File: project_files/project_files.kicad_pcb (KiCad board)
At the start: 2 copper layers, 142.9 x 95.2 mm, 27 parts, among them SW11 SW_Push, SW12 SW_Push, SW13 SW_Push, SW17 SW_Push, SW18 SW_Push, SW19 SW_Push, SW3 SW_Push, SW4 SW_Push, SW5 SW_Push, SW7 SW_Push, SW8 SW_Push, SW9 SW_Push, U1 MOUDLE-SEEEDUINO-XIAO

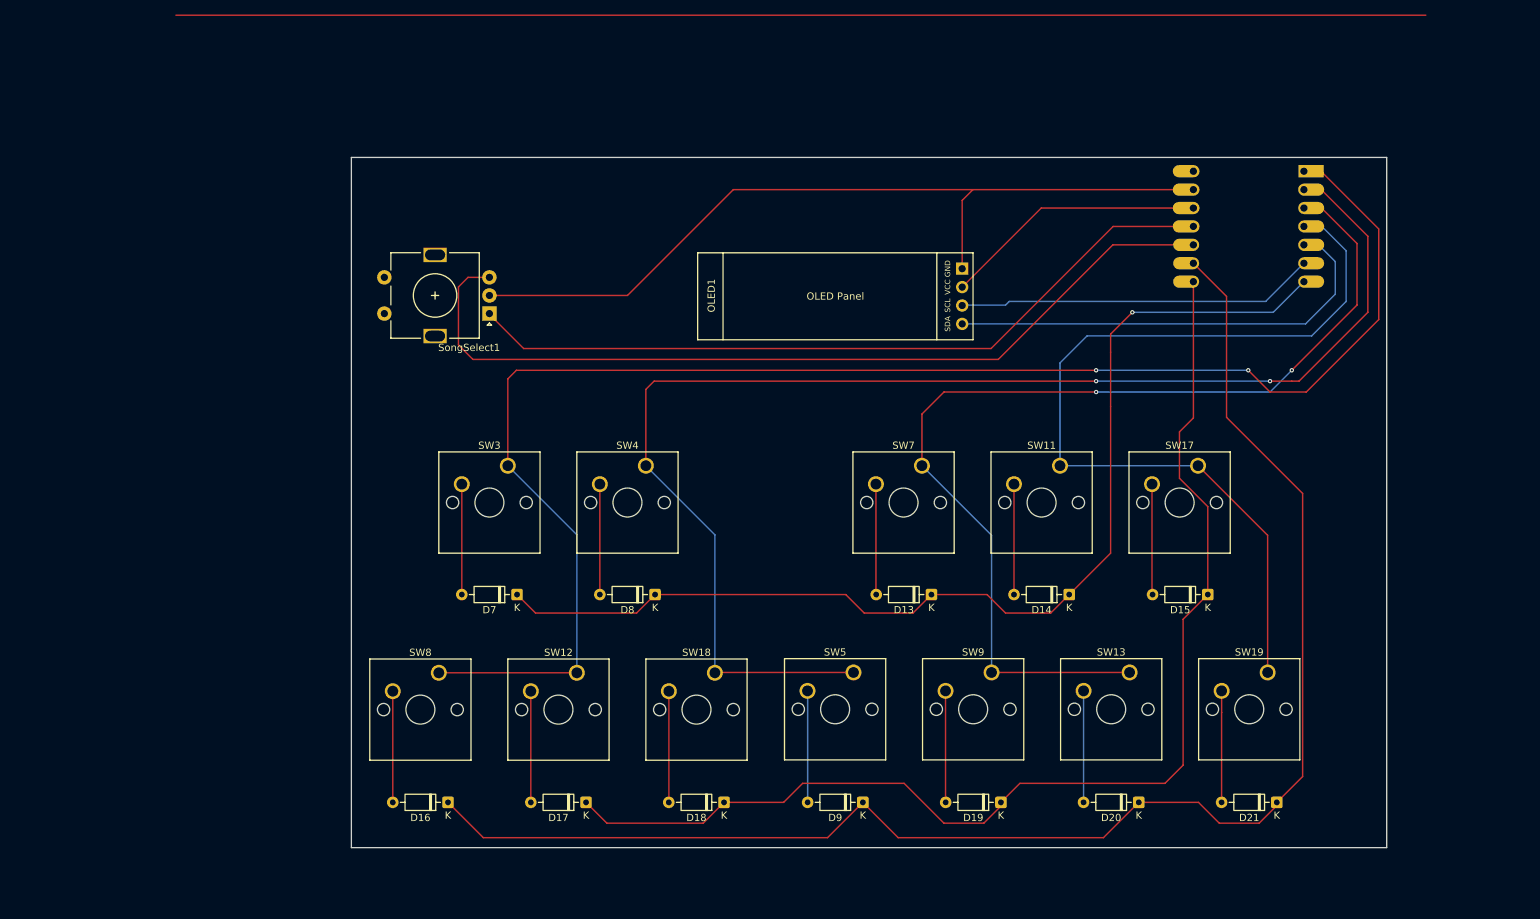
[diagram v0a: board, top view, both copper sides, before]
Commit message: new pcb design
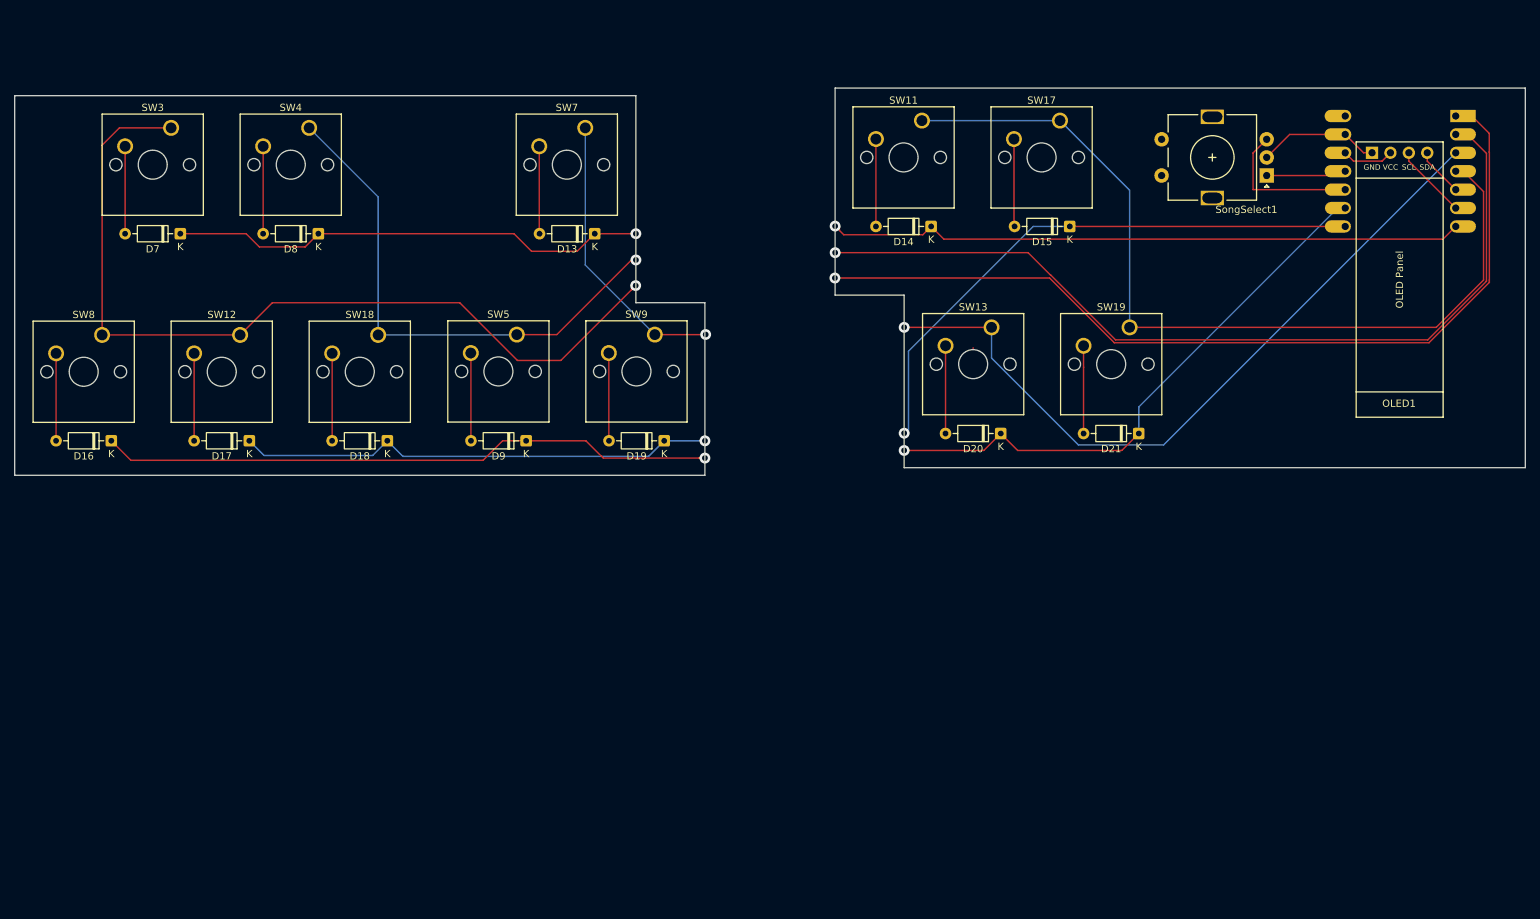
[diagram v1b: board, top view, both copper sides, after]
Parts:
- moved SongSelect1 108.9 mm to (212.0, 50.1)
- moved OLED1 93.7 mm to (224.4, 83.5), turned to 90 degrees
- moved D16 68.2 mm to (52.6, 86.7)
- moved D17 68.2 mm to (71.6, 86.7)
- moved D18 68.2 mm to (90.7, 86.7)
- moved D19 68.2 mm to (128.9, 86.7)
- moved D9 68.2 mm to (109.8, 86.7)
- moved D13 68.1 mm to (119.3, 58.2)
- moved D8 68.1 mm to (81.2, 58.2)
- moved D7 68.1 mm to (62.1, 58.2)
- moved SW12 65.8 mm to (70.4, 72.1)
- moved SW7 65.8 mm to (118.0, 43.5)
- moved SW8 65.8 mm to (51.3, 72.1)
- moved SW9 65.8 mm to (127.6, 72.1)
- moved SW3 65.8 mm to (60.9, 43.5)
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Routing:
- net /PIN_10: track 121.6 -> 21.3 mm
- net GND: track 114.7 -> 16.9 mm
- net /PIN_11: track 106.2 -> 11.2 mm
- net /SDA: track 63.0 -> 6.72 mm
- net /PIN_9: track 207.2 -> 163.2 mm, vias 0 -> 2
- net /SCL: track 49.6 -> 10.3 mm
- net /PWR_3v3: track 36.4 -> 7.19 mm
- net /PIN_1: track 215.7 -> 242.5 mm
- net /PIN_8: track 162.3 -> 145.0 mm, vias 0 -> 2
- net /PIN_2: track 188.2 -> 192.4 mm
- net /PIN_7: track 150.5 -> 154.1 mm, vias 1 -> 2
- net Net-(D21-A): track 15.4 -> 12.1 mm
- net Net-(D17-A): track 15.3 -> 12.1 mm
- net Net-(D16-A): track 15.3 -> 12.1 mm
- net Net-(D19-A): track 15.4 -> 12.1 mm
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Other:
- board size 142.9 x 95.2 mm -> 208.5 x 53.4 mm

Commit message: pcb done maybe
kudos anicetus
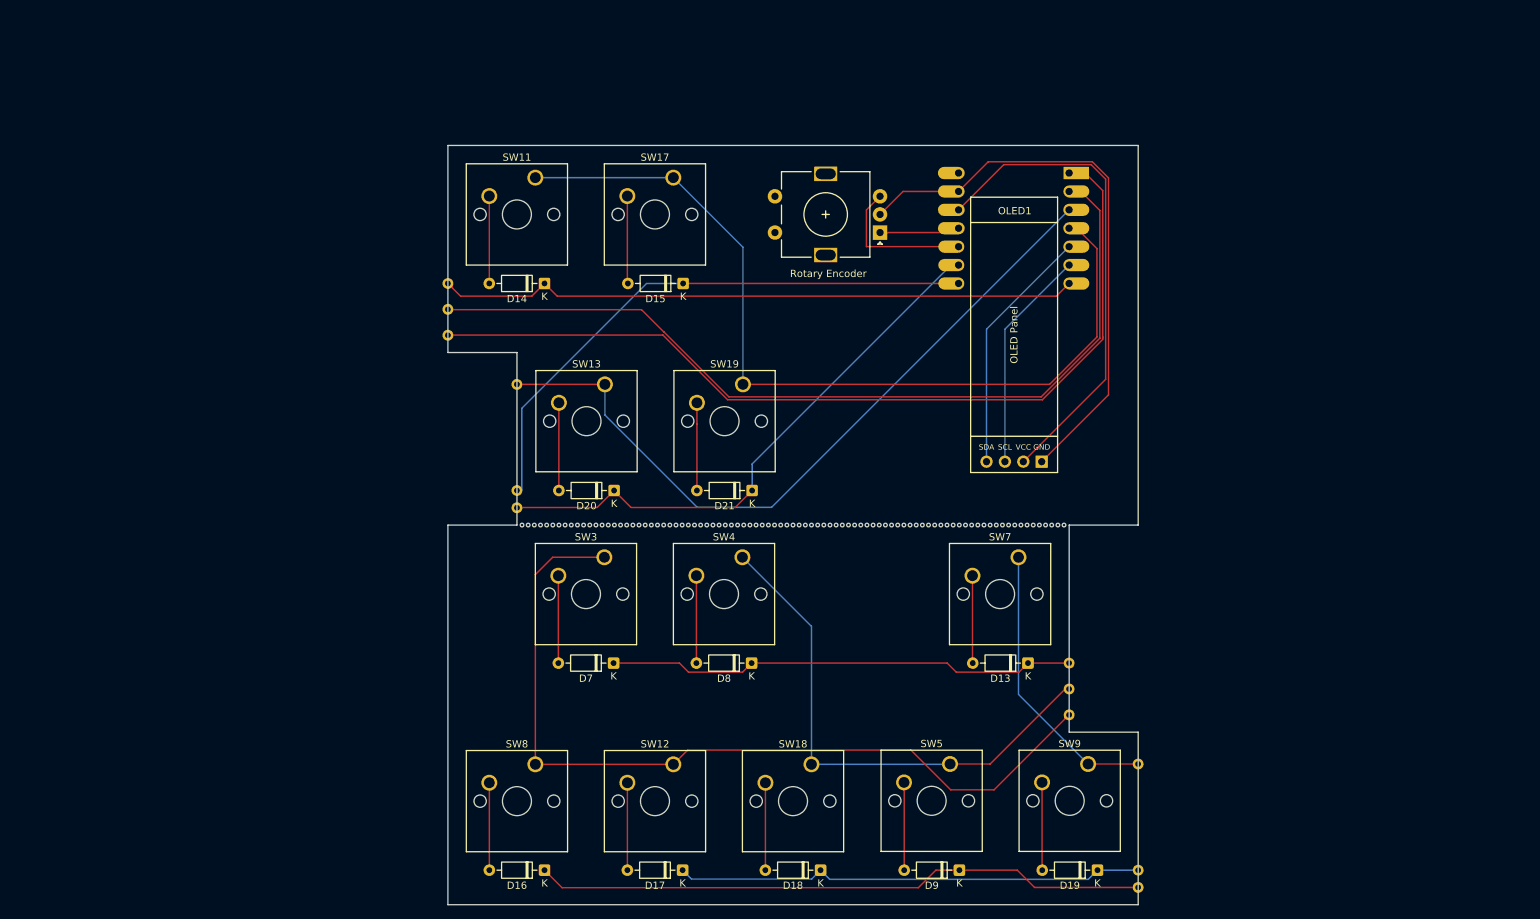
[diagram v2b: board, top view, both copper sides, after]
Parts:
- added ?: , , F.Cu at (99.0, 68.6)
- added ?: , , F.Cu at (108.6, 93.6)
- added ?: , , F.Cu at (108.6, 96.0)
- added ?: , , F.Cu at (194.3, 131.3)
- added ?: , , F.Cu at (184.8, 124.6)
- added ?: , , F.Cu at (194.3, 148.4)
- added ?: , , F.Cu at (99.0, 65.0)
- added ?: , , F.Cu at (184.8, 117.4)
- added ?: , , F.Cu at (194.3, 146.0)
- added ?: , , F.Cu at (184.8, 121.0)
- added ?: , , F.Cu at (108.6, 78.9)
- added ?: , , F.Cu at (99.0, 72.2)
- added REF**: BreakLine_11h_D0.5mm_P0.85mm, Panelization:BreakLine_11h_D0.5mm_P0.85mm, F.Cu at (179.0, 98.4)
- added REF**: BreakLine_11h_D0.5mm_P0.85mm, Panelization:BreakLine_11h_D0.5mm_P0.85mm, F.Cu at (132.2, 98.4)
- added REF**: BreakLine_11h_D0.5mm_P0.85mm, Panelization:BreakLine_11h_D0.5mm_P0.85mm, F.Cu at (113.5, 98.4)
- added REF**: BreakLine_11h_D0.5mm_P0.85mm, Panelization:BreakLine_11h_D0.5mm_P0.85mm, F.Cu at (141.6, 98.4)
- added REF**: BreakLine_11h_D0.5mm_P0.85mm, Panelization:BreakLine_11h_D0.5mm_P0.85mm, F.Cu at (122.9, 98.4)
- added REF**: BreakLine_1h_D0.5mm_P0.85mm, Panelization:BreakLine_1h_D0.5mm_P0.85mm, F.Cu at (184.1, 98.4)
- added REF**: BreakLine_11h_D0.5mm_P0.85mm, Panelization:BreakLine_11h_D0.5mm_P0.85mm, F.Cu at (169.6, 98.4)
- added REF**: BreakLine_11h_D0.5mm_P0.85mm, Panelization:BreakLine_11h_D0.5mm_P0.85mm, F.Cu at (160.3, 98.4)
- added REF**: BreakLine_11h_D0.5mm_P0.85mm, Panelization:BreakLine_11h_D0.5mm_P0.85mm, F.Cu at (150.9, 98.4)
- Rotary Encoder: renamed from SongSelect1
- moved D16 84.2 mm to (112.4, 146.0)
- moved D17 84.2 mm to (131.4, 146.0)
- moved D8 84.2 mm to (141.0, 117.4)
- moved SW5 84.2 mm to (168.3, 131.3)
- moved D7 84.2 mm to (121.9, 117.4)
- moved SW18 84.2 mm to (149.2, 131.4)
- moved SW3 84.2 mm to (120.6, 102.8)
- moved SW8 84.2 mm to (111.1, 131.4)
- moved D13 84.2 mm to (179.1, 117.4)
- moved D18 84.2 mm to (150.5, 146.0)
- moved D19 84.2 mm to (188.7, 146.0)
- moved D9 84.2 mm to (169.6, 146.0)
- moved SW12 84.2 mm to (130.2, 131.4)
- moved SW4 84.2 mm to (139.7, 102.8)
- moved SW7 84.2 mm to (177.8, 102.8)
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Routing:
- net GND: track 16.9 -> 78.4 mm
- net /PWR_3v3: track 7.19 -> 67.4 mm
- net /SDA: track 6.72 -> 34.4 mm
- net /SCL: track 10.3 -> 30.8 mm
- net /PIN_1: track 242.5 -> 238.3 mm, vias 2 -> 0
- net /PIN_8: track 145.0 -> 143.0 mm, vias 2 -> 0
- net /PIN_2: track 192.4 -> 190.7 mm, vias 2 -> 0
- net /PIN_9: track 163.2 -> 161.5 mm, vias 2 -> 0
- net /PIN_3: track 142.3 -> 140.9 mm, vias 2 -> 0
- net /PIN_7: track 154.1 -> 152.7 mm, vias 2 -> 0
- net /PIN_4: track 120.3 -> 119.3 mm
- net /PIN_11: track 11.2 -> 10.2 mm
- net /PIN_10: track 21.3 -> 20.4 mm
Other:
- board size 208.5 x 53.4 mm -> 95.3 x 104.8 mm
